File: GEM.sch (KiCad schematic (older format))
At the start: 0 parts

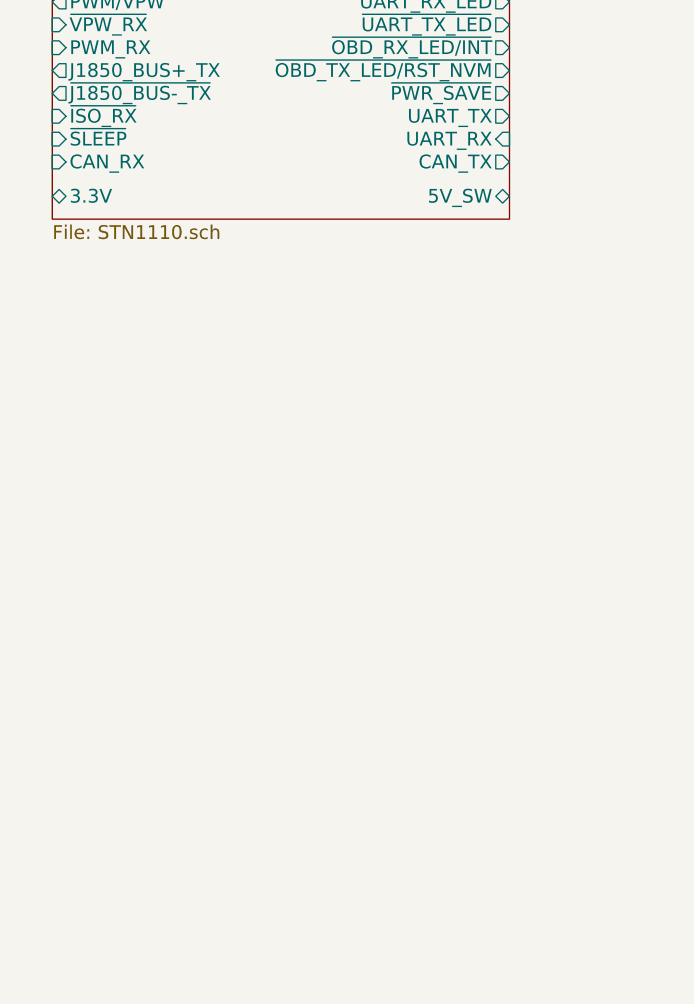
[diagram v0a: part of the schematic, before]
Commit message: Added MCP2551 and it's connections to STN1110
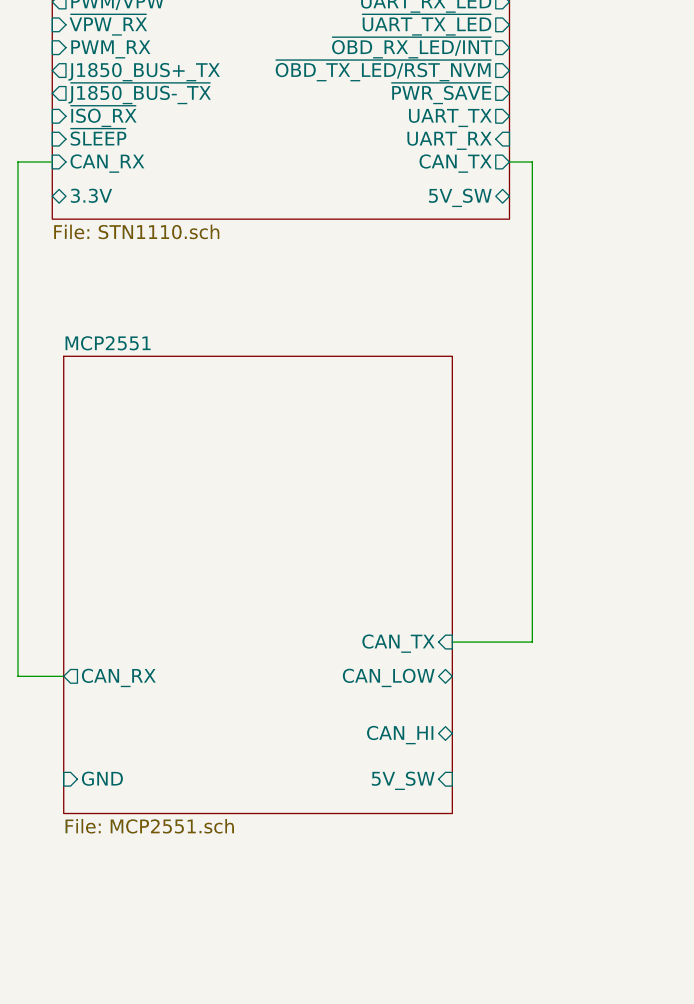
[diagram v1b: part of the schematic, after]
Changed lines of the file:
@@
 $Descr A4 11693 8268
 encoding utf-8
-Sheet 1 2
+Sheet 1 3
 Title ""
 Date ""
@@
 F24 "GND" B L 1300 1800 60
 $EndSheet
+$Sheet
+S 1350 3700 1700 2000
+U 5462582D
+F0 "MCP2551" 60
+F1 "MCP2551.sch" 60
+F2 "CAN_TX" I R 3050 4950 60
+F3 "CAN_RX" O L 1350 5100 60
+F4 "GND" I L 1350 5550 60
+F5 "5V_SW" I R 3050 5550 60
+F6 "CAN_HI" B R 3050 5350 60
+F7 "CAN_LOW" B R 3050 5100 60
+$EndSheet
+Wire Wire Line
+	1350 5100 1150 5100
+Wire Wire Line
+	1150 5100 1150 2850
+Wire Wire Line
+	1150 2850 1300 2850
+Wire Wire Line
+	3050 4950 3400 4950
+Wire Wire Line
+	3400 4950 3400 2850
+Wire Wire Line
+	3400 2850 3300 2850
 $EndSCHEMATC

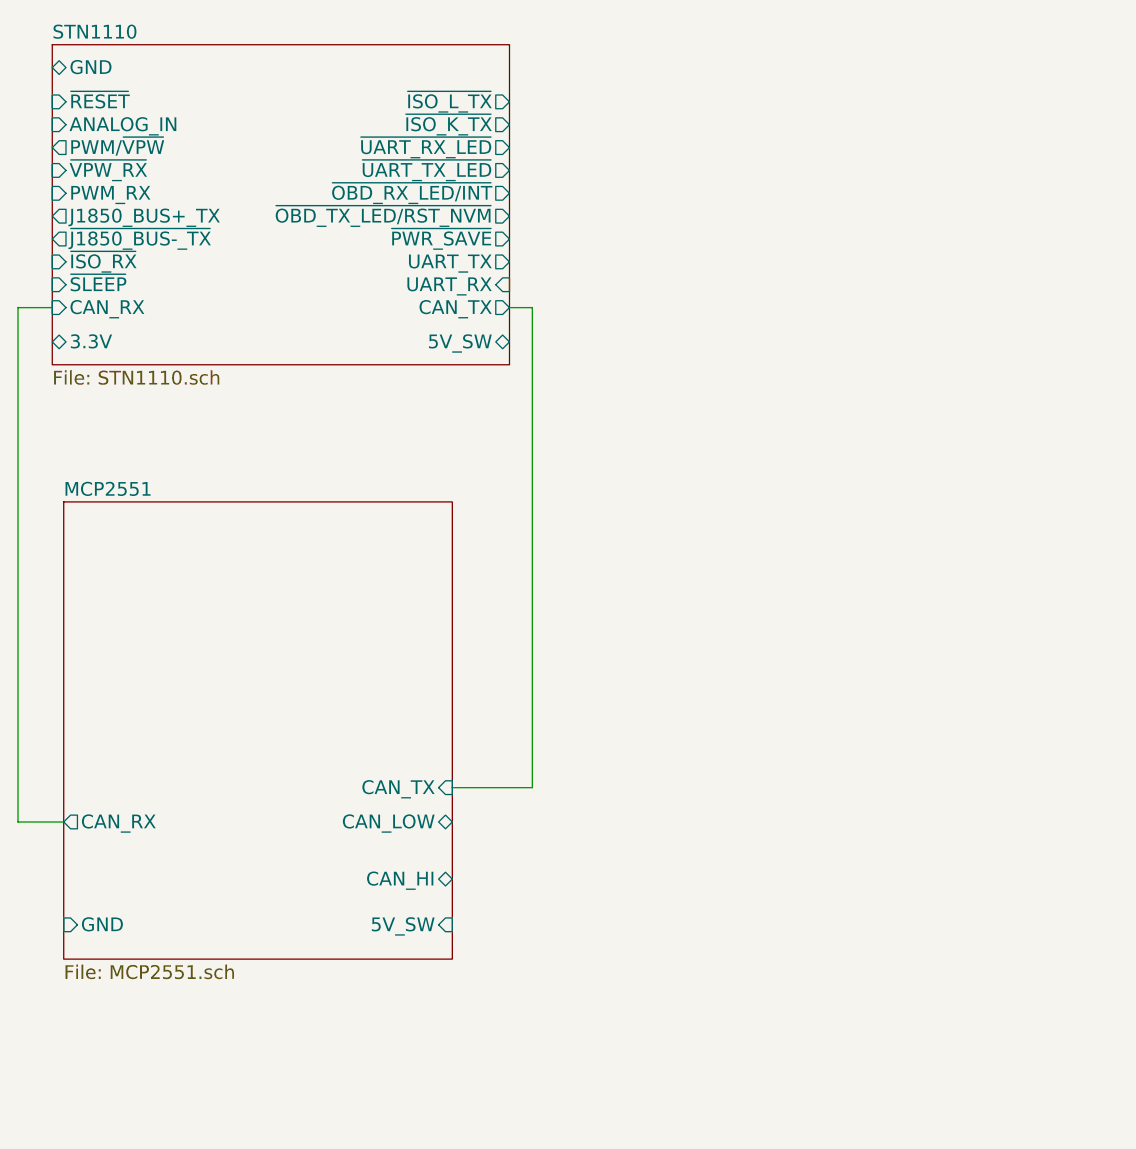
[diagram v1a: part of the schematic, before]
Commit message: Added status lights sheet
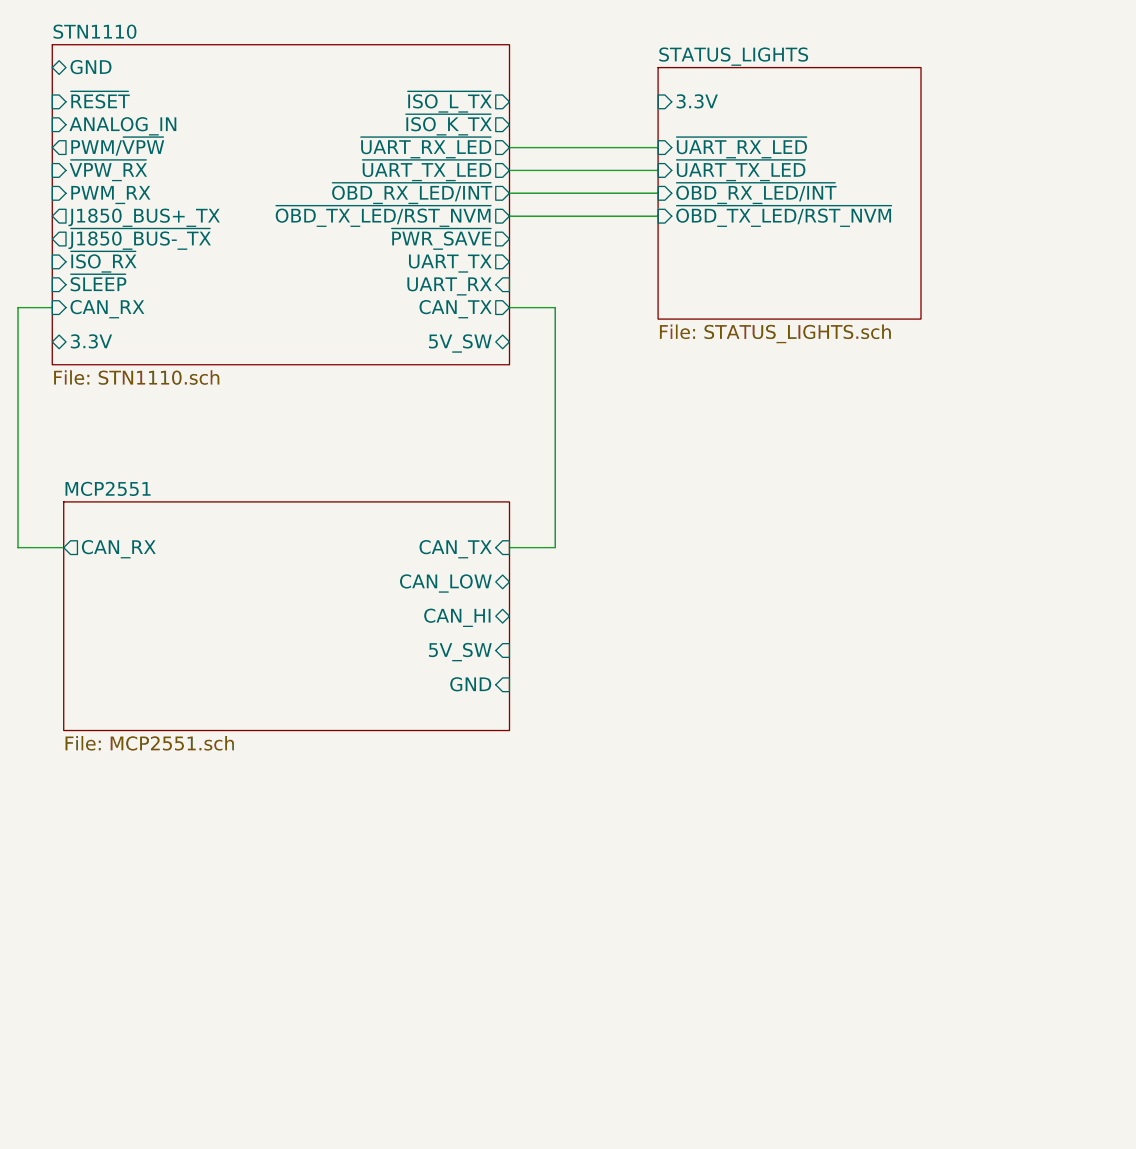
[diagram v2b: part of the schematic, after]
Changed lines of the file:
@@
 $Descr A4 11693 8268
 encoding utf-8
-Sheet 1 3
+Sheet 1 4
 Title ""
 Date ""
@@
 $EndSheet
 $Sheet
-S 1350 3700 1700 2000
+S 1350 3700 1950 1000
 U 5462582D
 F0 "MCP2551" 60
 F1 "MCP2551.sch" 60
-F2 "CAN_TX" I R 3050 4950 60
-F3 "CAN_RX" O L 1350 5100 60
-F4 "GND" I L 1350 5550 60
-F5 "5V_SW" I R 3050 5550 60
-F6 "CAN_HI" B R 3050 5350 60
-F7 "CAN_LOW" B R 3050 5100 60
+F2 "CAN_TX" I R 3300 3900 60
+F3 "CAN_RX" O L 1350 3900 60
+F4 "GND" I R 3300 4500 60
+F5 "5V_SW" I R 3300 4350 60
+F6 "CAN_HI" B R 3300 4200 60
+F7 "CAN_LOW" B R 3300 4050 60
 $EndSheet
-Wire Wire Line
-	1350 5100 1150 5100
-Wire Wire Line
-	1150 5100 1150 2850
 Wire Wire Line
 	1150 2850 1300 2850
 Wire Wire Line
-	3050 4950 3400 4950
+	3300 2850 3500 2850
 Wire Wire Line
-	3400 4950 3400 2850
+	1150 2850 1150 3900
 Wire Wire Line
-	3400 2850 3300 2850
+	1150 3900 1350 3900
+Wire Wire Line
+	3300 3900 3500 3900
+Wire Wire Line
+	3500 3900 3500 2850
+$Sheet
+S 3950 1800 1150 1100
+U 5462AB81
+F0 "STATUS_LIGHTS" 60
+F1 "STATUS_LIGHTS.sch" 60
+F2 "3.3V" I L 3950 1950 60
+F3 "~OBD_TX_LED/RST_NVM" I L 3950 2450 60
+F4 "~OBD_RX_LED/INT" I L 3950 2350 60
+F5 "~UART_TX_LED" I L 3950 2250 60
+F6 "~UART_RX_LED" I L 3950 2150 60
+$EndSheet
+Wire Wire Line
+	3300 2150 3950 2150
+Wire Wire Line
+	3300 2250 3950 2250
+Wire Wire Line
+	3300 2350 3950 2350
+Wire Wire Line
+	3300 2450 3950 2450
 $EndSCHEMATC
